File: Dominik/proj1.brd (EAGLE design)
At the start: 125.4 x 78.7 mm, 18 parts, among them IC1 PCF8574P, U1 ATMEGA328P_PDIP

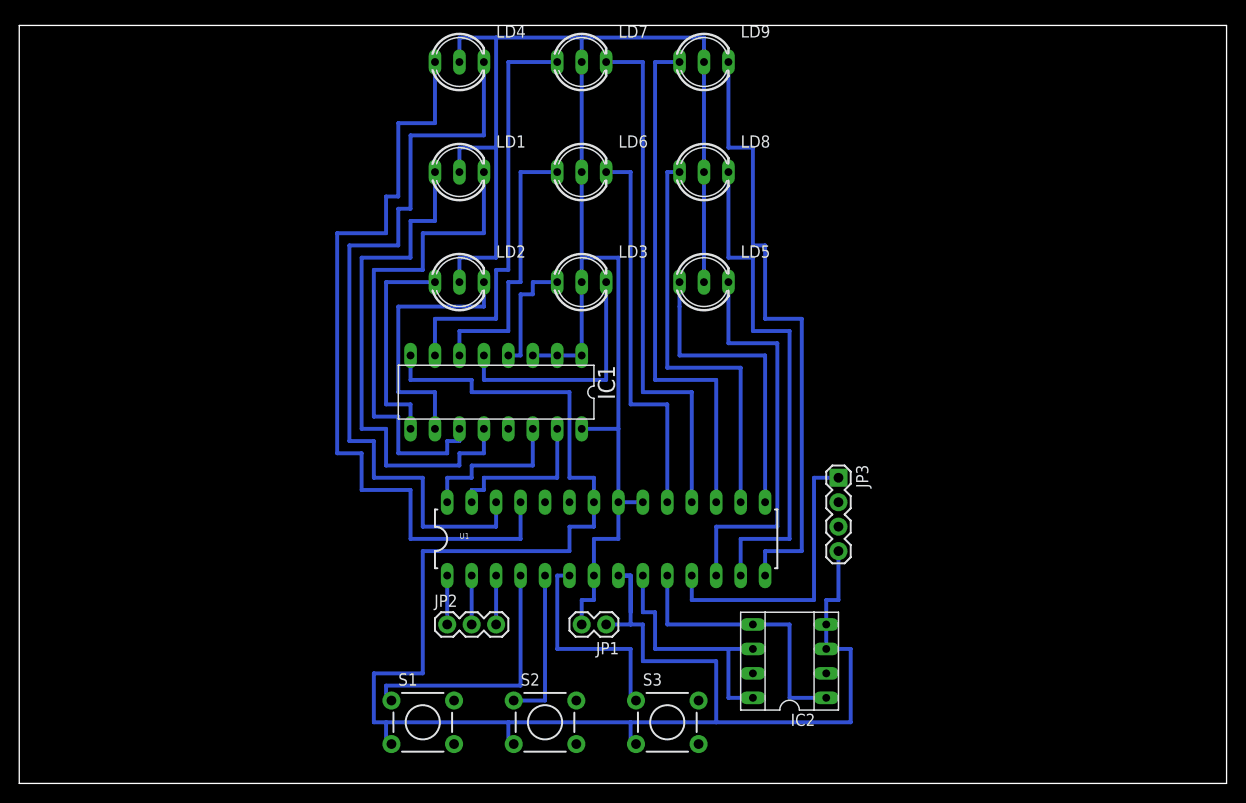
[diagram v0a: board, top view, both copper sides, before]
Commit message: final version
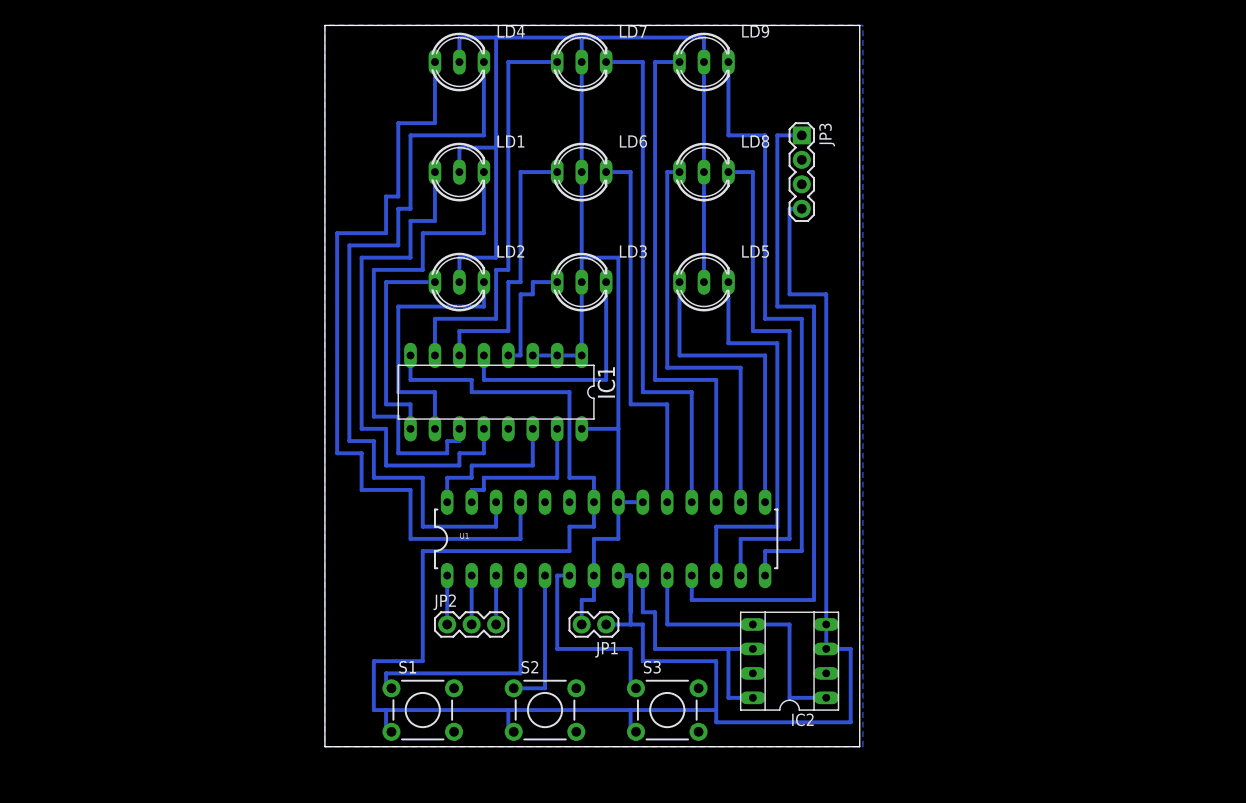
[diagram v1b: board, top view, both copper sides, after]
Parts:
- moved JP3 35.8 mm to (92.7, 66.0)
- moved S1 1.27 mm to (53.3, 6.35)
- moved S2 1.27 mm to (66.0, 6.35)
- moved S3 1.27 mm to (78.7, 6.35)
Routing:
- net N$10: track 30.5 -> 69.8 mm
- net N$32: track 177.4 -> 215.5 mm
- net N$1: track 27.5 -> 26.2 mm
- net N$14: track 16.2 -> 15.0 mm
- net N$15: track 22.4 -> 21.2 mm
- added copper zone on layer 16, net S$11
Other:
- board size 125.4 x 78.7 mm -> 55.6 x 74.9 mm

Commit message: added tictactoe design
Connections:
- net N$1 renamed BTN0
- net N$10 renamed PIEZO
- net N$14 renamed BTN1
- net N$15 renamed BTN2
- net N$18 renamed LED5_1
- net N$19 renamed LED8_1
- net N$20 renamed LED5_2
- net N$21 renamed LED2_2
- net N$22 renamed LED0_1
- net N$24 renamed LED3_1
- net N$25 renamed LED4_2
- net N$26 renamed LED8_2
- net N$28 renamed LED1_1
- net N$3 renamed LED0_2
- net N$31 renamed LED3_2
- net S$1 renamed LED4_1
- net S$13 renamed LED1_2
- net S$3 renamed LED6_2
- net S$4 renamed LED7_2
- net S$5 renamed LED6_1
- net S$6 renamed LED7_1
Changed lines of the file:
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@@
 <wire x1="58.42" y1="15.24" x2="58.42" y2="20.32" width="0.4064" layer="16"/>
 </signal>
-<signal name="N$3">
+<signal name="LED0_2">
 <contactref element="LD4" pad="AR"/>
 <wire x1="59.69" y1="73.66" x2="59.69" y2="66.04" width="0.4064" layer="16"/>
@@
 <wire x1="87.63" y1="15.24" x2="78.74" y2="15.24" width="0.4064" layer="16"/>
 </signal>
-<signal name="N$1">
+<signal name="BTN0">
 <contactref element="U1" pad="4"/>
 <contactref element="S1" pad="1"/>
@@
 <wire x1="74.93" y1="15.24" x2="76.2" y2="15.24" width="0.4064" layer="16"/>
 </signal>
-<signal name="N$14">
+<signal name="BTN1">
 <contactref element="S2" pad="1"/>
 <contactref element="U1" pad="5"/>
@@
 <wire x1="66.04" y1="8.6106" x2="66.04" y2="20.32" width="0.4064" layer="16"/>
 </signal>
-<signal name="N$15">
+<signal name="BTN2">
 <contactref element="U1" pad="6"/>
 <contactref element="S3" pad="1"/>
@@
 <wire x1="77.47" y1="73.66" x2="80.01" y2="73.66" width="0.4064" layer="16"/>
 </signal>
-<signal name="N$18">
+<signal name="LED5_1">
 <contactref element="U1" pad="16"/>
 <wire x1="86.36" y1="27.94" x2="86.36" y2="41.91" width="0.4064" layer="16"/>
@@
 <wire x1="80.01" y1="62.23" x2="78.74" y2="62.23" width="0.4064" layer="16"/>
 </signal>
-<signal name="N$19">
+<signal name="LED8_1">
 <contactref element="U1" pad="15"/>
 <wire x1="88.9" y1="27.94" x2="88.9" y2="43.18" width="0.4064" layer="16"/>
@@
 <contactref element="LD5" pad="AX"/>
 </signal>
-<signal name="N$20">
+<signal name="LED5_2">
 <contactref element="LD8" pad="AR"/>
 <wire x1="86.36" y1="24.13" x2="91.44" y2="24.13" width="0.4064" layer="16"/>
@@
 <wire x1="87.63" y1="62.23" x2="85.09" y2="62.23" width="0.4064" layer="16"/>
 </signal>
-<signal name="N$21">
+<signal name="LED2_2">
 <contactref element="LD9" pad="AR"/>
 <wire x1="88.9" y1="22.86" x2="92.71" y2="22.86" width="0.4064" layer="16"/>
@@
 <wire x1="60.96" y1="20.32" x2="60.96" y2="15.24" width="0.4064" layer="16"/>
 </signal>
-<signal name="N$22">
+<signal name="LED0_1">
 <contactref element="LD4" pad="AX"/>
 <contactref element="U1" pad="25"/>
@@
 <wire x1="54.61" y1="67.31" x2="54.61" y2="73.66" width="0.4064" layer="16"/>
 </signal>
-<signal name="N$24">
+<signal name="LED3_1">
 <contactref element="LD1" pad="AX"/>
 <wire x1="46.99" y1="35.56" x2="46.99" y2="53.34" width="0.4064" layer="16"/>
@@
 <wire x1="54.61" y1="57.15" x2="54.61" y2="62.23" width="0.4064" layer="16"/>
 </signal>
-<signal name="N$25">
+<signal name="LED4_2">
 <contactref element="LD6" pad="AR"/>
 <wire x1="72.39" y1="62.23" x2="74.93" y2="62.23" width="0.4064" layer="16"/>
@@
 <wire x1="78.74" y1="38.1" x2="78.74" y2="27.94" width="0.4064" layer="16"/>
 </signal>
-<signal name="N$26">
+<signal name="LED8_2">
 <contactref element="LD5" pad="AR"/>
 <wire x1="83.82" y1="25.4" x2="90.17" y2="25.4" width="0.4064" layer="16"/>
@@
 <wire x1="85.09" y1="44.45" x2="85.09" y2="50.8" width="0.4064" layer="16"/>
 </signal>
-<signal name="S$3">
+<signal name="LED6_2">
 <wire x1="50.8" y1="48.26" x2="59.69" y2="48.26" width="0.4064" layer="16"/>
 <contactref element="LD2" pad="AR"/>
@@
 <wire x1="54.61" y1="39.37" x2="54.61" y2="35.56" width="0.4064" layer="16"/>
 </signal>
-<signal name="S$13">
+<signal name="LED1_2">
 <wire x1="76.2" y1="39.37" x2="76.2" y2="73.66" width="0.4064" layer="16"/>
 <wire x1="81.28" y1="39.37" x2="76.2" y2="39.37" width="0.4064" layer="16"/>
@@
 <wire x1="76.2" y1="73.66" x2="72.39" y2="73.66" width="0.4064" layer="16"/>
 </signal>
-<signal name="N$28">
+<signal name="LED1_1">
 <contactref element="IC1" pad="7"/>
 <wire x1="54.61" y1="43.18" x2="54.61" y2="46.99" width="0.4064" layer="16"/>
@@
 <wire x1="62.23" y1="52.07" x2="62.23" y2="73.66" width="0.4064" layer="16"/>
 </signal>
-<signal name="N$31">
+<signal name="LED3_2">
 <contactref element="IC1" pad="11"/>
 <wire x1="57.15" y1="34.29" x2="57.15" y2="35.56" width="0.4064" layer="16"/>
@@
 <wire x1="95.25" y1="49.53" x2="95.25" y2="15.24" width="0.4064" layer="16"/>
 </signal>
-<signal name="N$10">
+<signal name="PIEZO">
 <contactref element="U1" pad="11"/>
 <wire x1="93.98" y1="17.78" x2="81.28" y2="17.78" width="0.4064" layer="16"/>
@@
 <wire x1="90.17" y1="48.26" x2="93.98" y2="48.26" width="0.4064" layer="16"/>
 </signal>
-<signal name="S$1">
+<signal name="LED4_1">
 <contactref element="IC1" pad="6"/>
 <wire x1="57.15" y1="43.18" x2="57.15" y2="45.72" width="0.4064" layer="16"/>
@@
 <wire x1="62.23" y1="45.72" x2="62.23" y2="50.8" width="0.4064" layer="16"/>
 </signal>
-<signal name="S$4">
+<signal name="LED7_2">
 <contactref element="IC1" pad="5"/>
 <wire x1="59.69" y1="43.18" x2="59.69" y2="40.64" width="0.4064" layer="16"/>
@@
 <wire x1="67.31" y1="30.48" x2="67.31" y2="35.56" width="0.4064" layer="16"/>
 </signal>
-<signal name="S$6">
+<signal name="LED7_1">
 <contactref element="IC1" pad="4"/>
 <wire x1="62.23" y1="43.18" x2="63.5" y2="43.18" width="0.4064" layer="16"/>
@@
 <wire x1="64.77" y1="50.8" x2="67.31" y2="50.8" width="0.4064" layer="16"/>
 </signal>
-<signal name="S$5">
+<signal name="LED6_1">
 <contactref element="LD2" pad="AX"/>
 <wire x1="54.61" y1="50.8" x2="49.53" y2="50.8" width="0.4064" layer="16"/>
